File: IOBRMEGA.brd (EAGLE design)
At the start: 86.4 x 53.3 mm, 20 parts, among them J1 Digital_0_7, J10 Power, J11 M06X2-SHROUDED, J12 M06X2-SHROUDED, J13 M06X2-SHROUDED, J14 M06X2-SHROUDED, J15 M06X2-SHROUDED, J16 M06X2-SHROUDED, J17 M06X2-SHROUDED, J18 M06X2-SHROUDED, J19 ICSP:MAIN, J2 Analog_0_7, J3 Digital_8_13, J4 Analog_8_15, J5 Digital_14_21, J6 Digital_22_36, J7 Digital_23_37, J8 Digital_38_52, J9 Digital_39_53

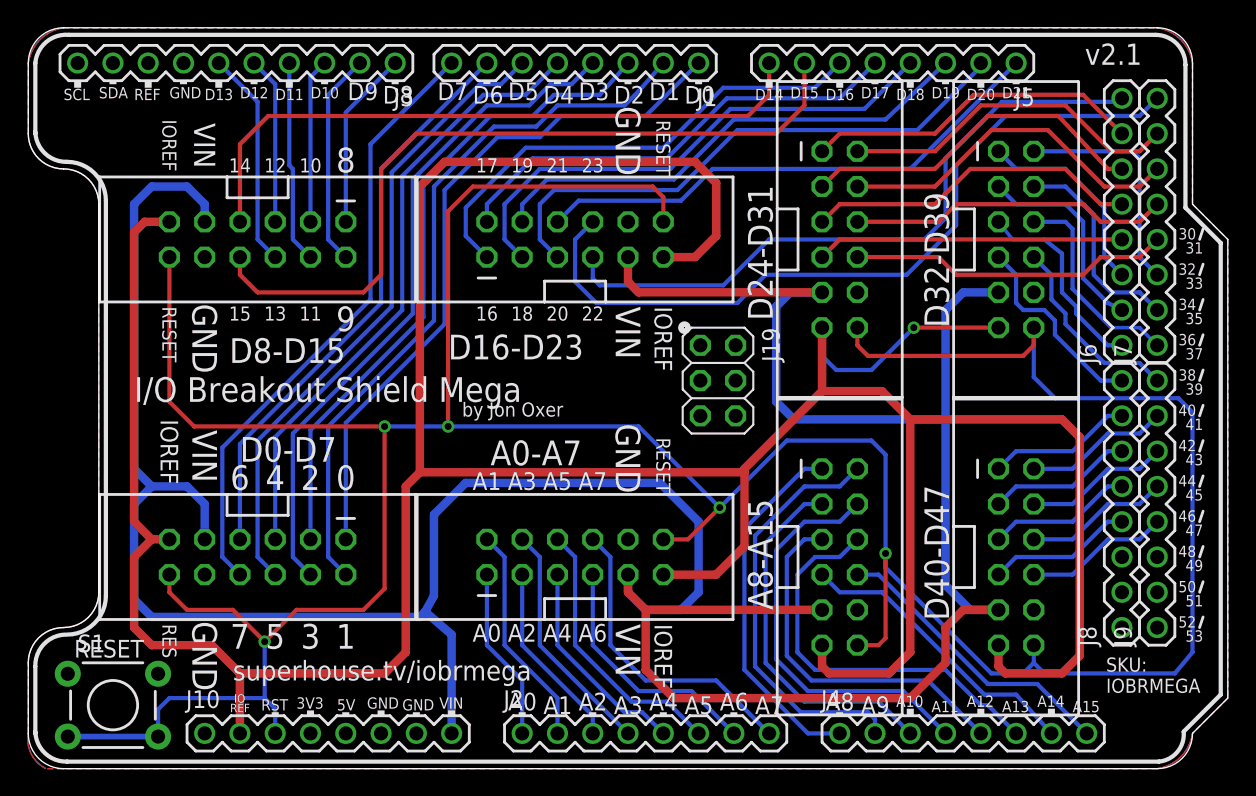
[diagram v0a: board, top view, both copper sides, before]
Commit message: Final tweaks for v2.1 release
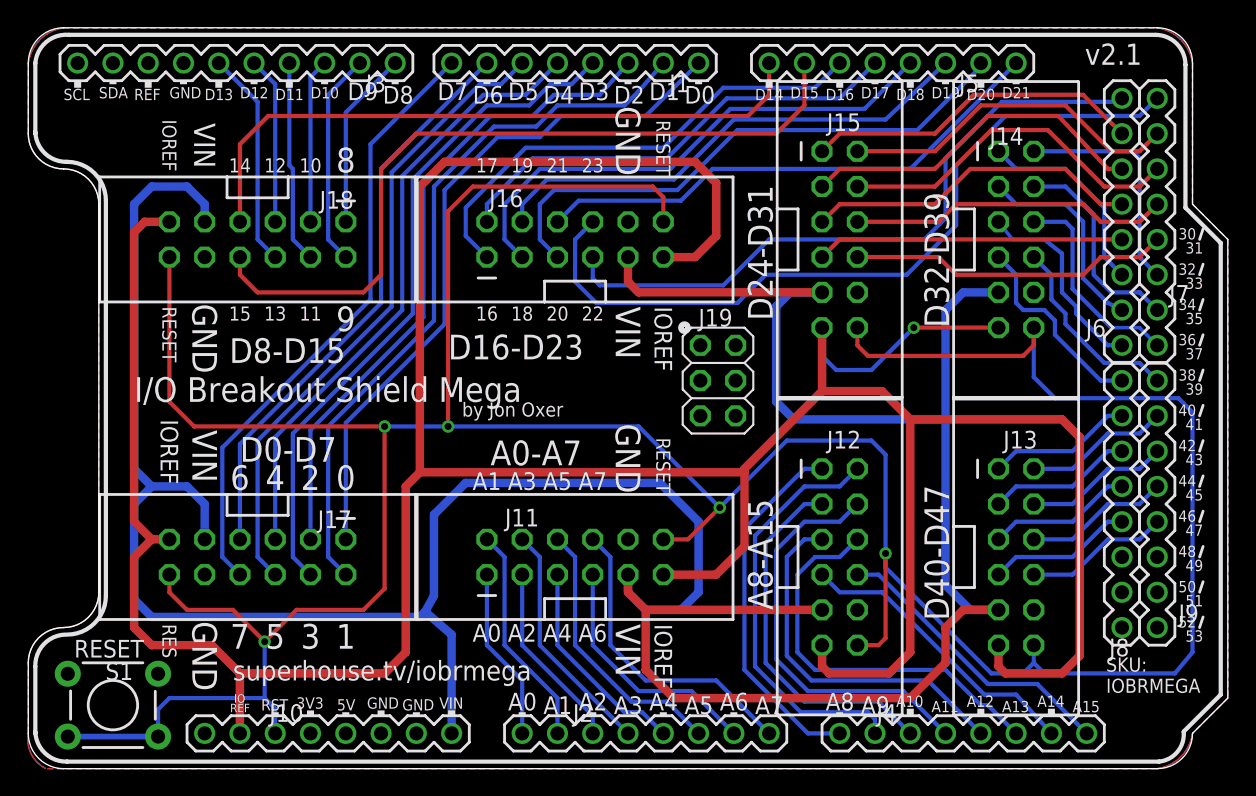
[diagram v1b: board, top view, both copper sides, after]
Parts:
- J11, J12, J13, J14, J15, J16, J17, J18: value M06X2-SHROUDED -> M02X6-SHROUDED; device SuperHouse-Connectors:2X6-SHROUDED -> SuperHouse-Connectors:2X06-SHROUDED
